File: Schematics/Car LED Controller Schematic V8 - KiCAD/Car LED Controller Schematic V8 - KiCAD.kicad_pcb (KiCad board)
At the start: 2 copper layers, 101.9 x 70 mm, 20 parts, among them J1 5V Power In, J2 Select Button, J3 LCD, Relay, LED Signal, J4 ZSS-108-01-F-D-506, J5 DRL, Horn Sense, U1 ESP32-DEVKITC-32D, U2 BOB-12009

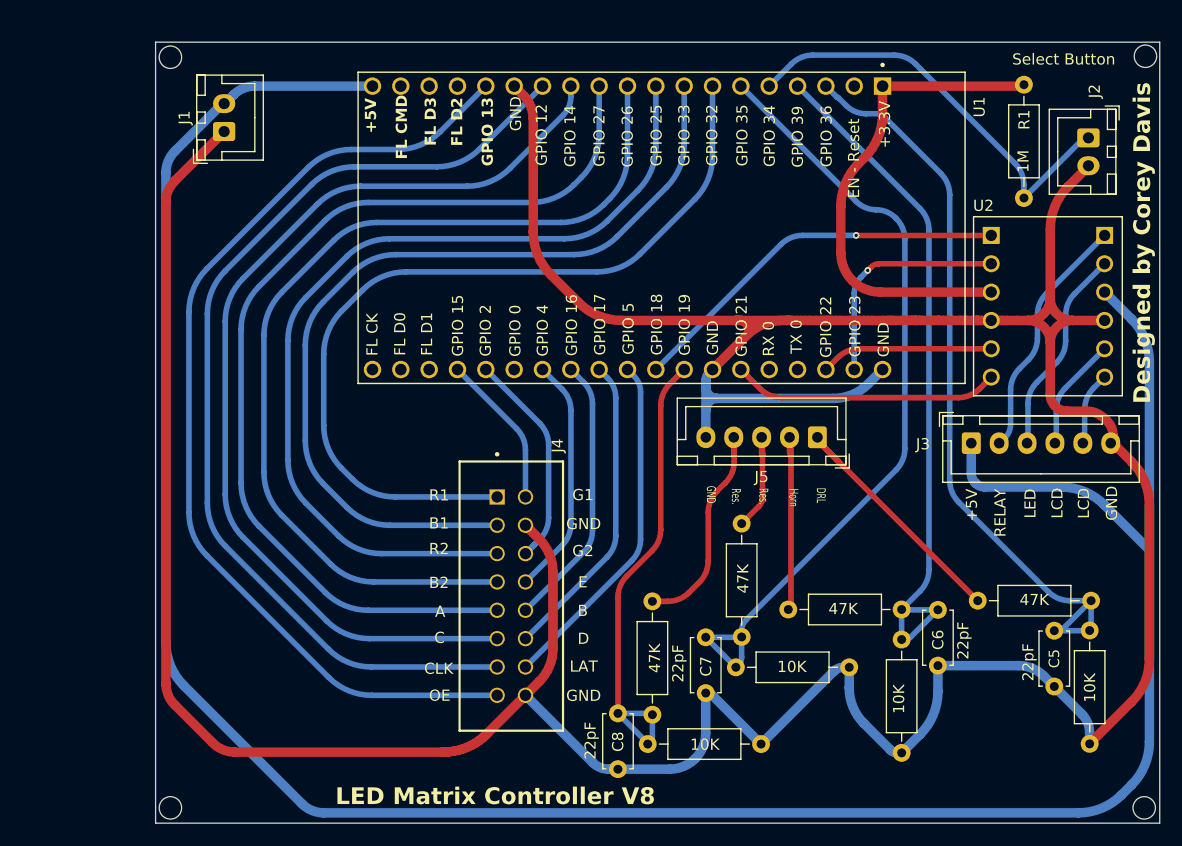
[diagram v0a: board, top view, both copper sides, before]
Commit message: more pcb
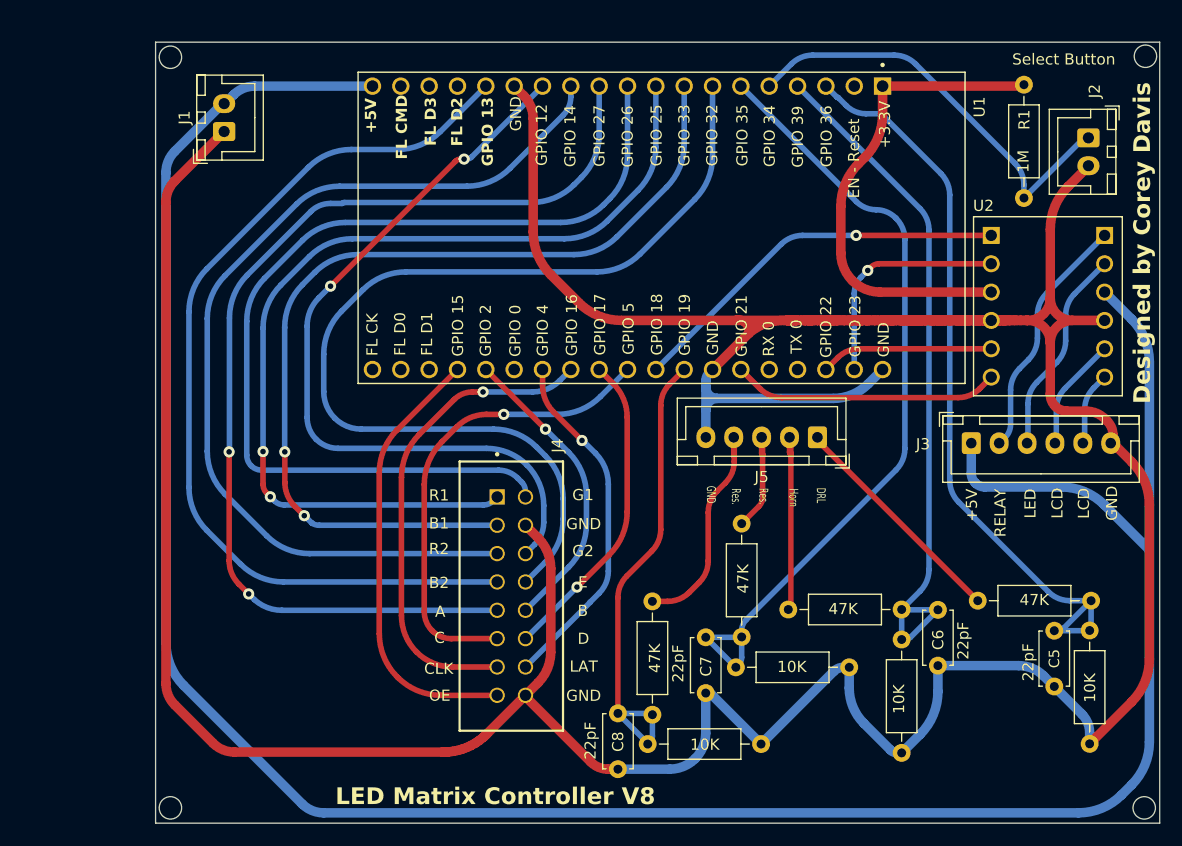
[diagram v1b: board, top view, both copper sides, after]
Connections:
- J4 pad 02: /Net-(J4-LAT) -> Net-(J4-G1)
- J4 pad 06: /Net-(J4-D) -> Net-(J4-G2)
- J4 pad 08: /Net-(J4-B) -> Net-(J4-E)
- J4 pad 10: /Net-(J4-E) -> Net-(J4-B)
- J4 pad 14: /Net-(J4-G1) -> Net-(J4-LAT)
- U1 pad J2-10: Net-(J4-B2) -> Net-(J4-G1)
- U1 pad J2-12: Net-(J4-C) -> Net-(J4-R2)
- U1 pad J2-13: Net-(J4-CLK) -> Net-(J4-G2)
- U1 pad J2-15: Net-(J4-OE) -> Net-(J4-B2)
- U1 pad J2-7: Net-(J4-R1) -> Net-(J4-E)
- U1 pad J2-9: Net-(J4-R2) -> Net-(J4-R1)
- U1 pad J3-10: /Net-(J4-G1) -> Net-(J4-C)
- U1 pad J3-12: /Net-(J4-E) -> Net-(J4-CLK)
- U1 pad J3-13: /Net-(J4-B) -> Net-(J4-LAT)
- U1 pad J3-15: /Net-(J4-D) -> Net-(J4-B)
- U1 pad J3-16: /Net-(J4-LAT) -> Net-(J4-OE)
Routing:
- net Net-(J4-E): track 0.00 -> 88.8 mm
- net Net-(J4-G1): track 0.00 -> 87.2 mm
- net Net-(J4-G2): track 0.00 -> 69.3 mm, vias 0 -> 2
- net Net-(J4-OE): track 88.7 -> 40.0 mm
- net Net-(J4-CLK): track 88.8 -> 43.5 mm, vias 0 -> 1
- net Net-(J4-C): track 87.3 -> 42.4 mm, vias 0 -> 1
- net Net-(J4-LAT): track 0.00 -> 31.7 mm, vias 0 -> 1
- net /Net-(J4-G1): track 31.2 -> 0.00 mm
- net Net-(J4-B): track 0.00 -> 27.1 mm, vias 0 -> 1
- net /Net-(J4-E): track 24.6 -> 0.00 mm
- net /Net-(J4-B): track 21.5 -> 0.00 mm
- net /Net-(J4-D): track 19.4 -> 0.00 mm
- net /Net-(J4-LAT): track 13.8 -> 0.00 mm
- net Net-(J4-R1): track 75.5 -> 85.1 mm, vias 0 -> 2
- net Net-(J4-A): track 87.5 -> 94.0 mm, vias 0 -> 2
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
